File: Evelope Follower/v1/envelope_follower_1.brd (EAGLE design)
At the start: 160 x 100 mm, 18 parts, among them J1 MJ-3536N, J2 MJ-3536N, J3 OSTVN03A150

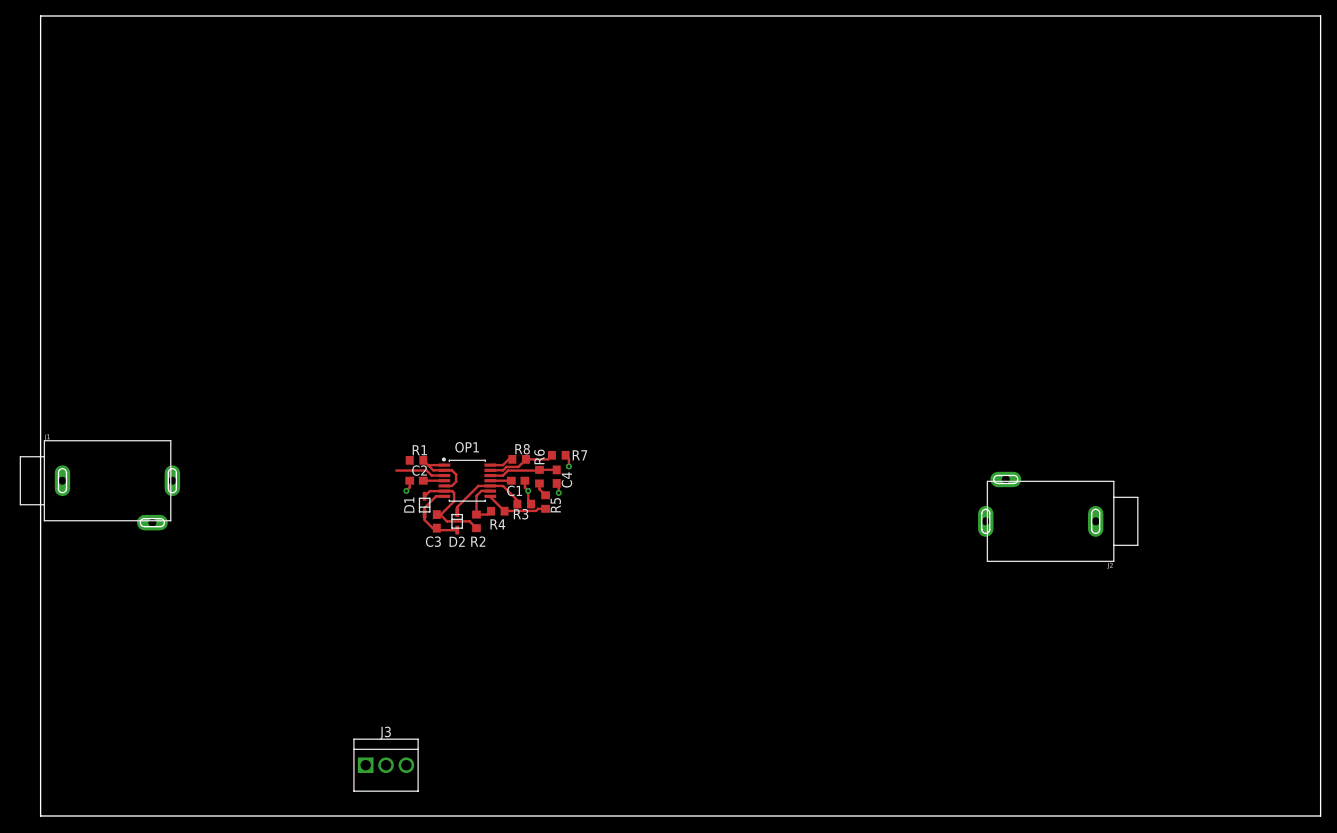
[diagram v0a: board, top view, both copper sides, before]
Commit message: more changes
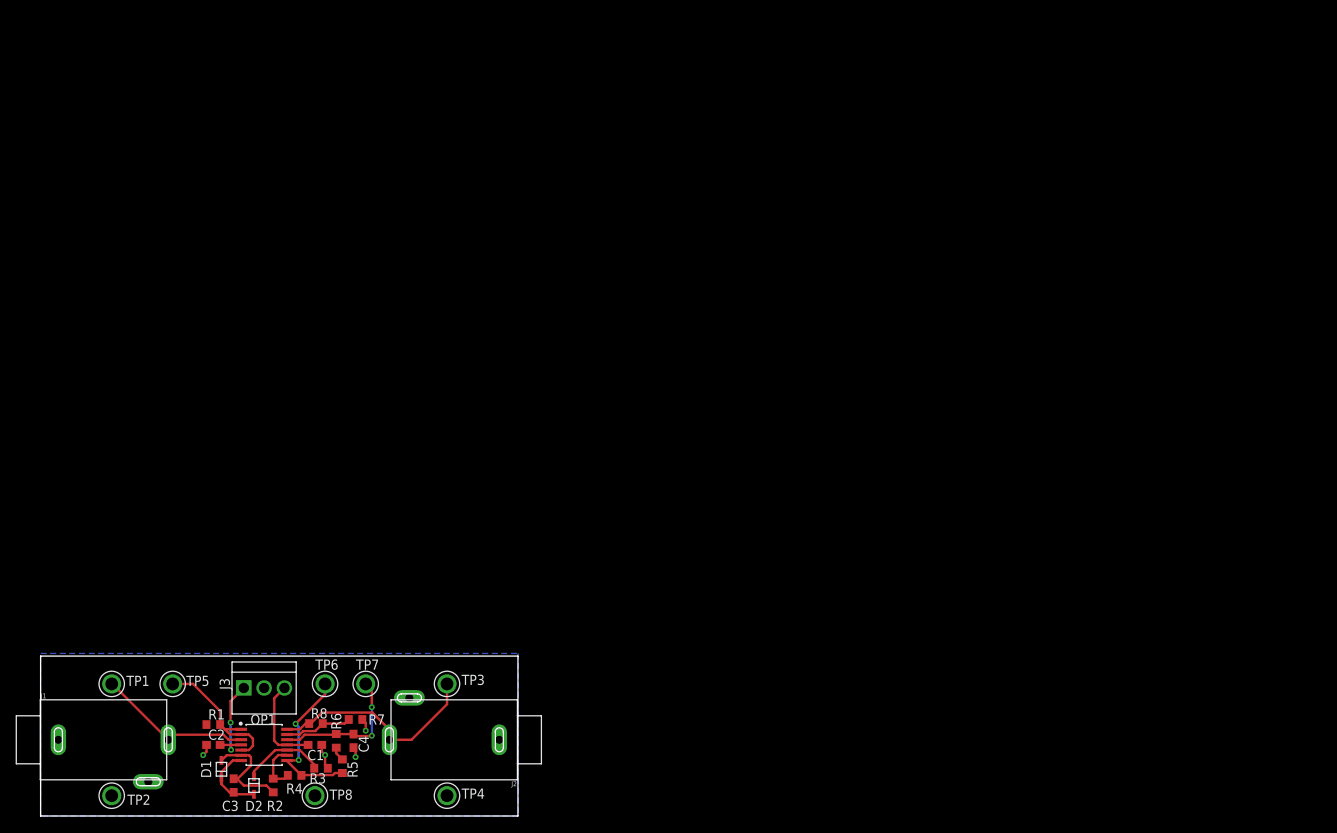
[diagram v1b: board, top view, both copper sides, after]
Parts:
- added TP1, TP2, TP3, TP4, TP5, TP6, TP7, TP8: (no value), roomready:TP_THM_1.6_S
- moved J2 79.4 mm to (46.1, 9.53)
- moved C2 41.7 mm to (21.6, 8.89)
- moved C3 41.7 mm to (24.1, 3.81)
- moved C4 41.7 mm to (39.1, 9.40)
- moved D1 41.7 mm to (22.6, 5.84)
- moved OP1 41.7 mm to (27.9, 8.89)
- moved R1 41.7 mm to (21.6, 11.4)
- moved R4 41.7 mm to (31.8, 5.08)
- moved R5 41.7 mm to (37.7, 6.22)
- moved R7 41.7 mm to (39.4, 12.1)
- moved C1 41.7 mm to (34.3, 8.89)
- moved D2 41.7 mm to (26.7, 3.81)
- moved R2 41.7 mm to (29.1, 3.81)
- moved R3 41.7 mm to (35.1, 5.97)
- moved R6 41.7 mm to (37.0, 9.40)
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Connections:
- net ENV: now also TP3.P$1
- net GND: now also TP2.P$1, TP4.P$1, TP8.P$1
- net LP_FILT: now also TP7.P$1
- net RECT: now also TP6.P$1
- net SRC: now also TP1.P$1
- net SRC_BUFF: now also TP5.P$1
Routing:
- net ENV: track 3.05 -> 27.4 mm
- net SRC: track 6.28 -> 19.6 mm
- net RECT: track 7.84 -> 20.5 mm, vias 0 -> 2
- net LP_FILT: track 8.61 -> 17.8 mm, vias 0 -> 2
- net +12V: track 2.63 -> 11.7 mm, vias 0 -> 2
- net SRC_BUFF: track 9.46 -> 18.5 mm
- net -12V: track 2.63 -> 11.6 mm
- added copper zone on layer 16, net GND
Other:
- board size 160 x 100 mm -> 59.7 x 20 mm
